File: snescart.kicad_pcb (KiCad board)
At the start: 2 copper layers, 101.6 x 37.3 mm, 7 parts, among them P1 CASSETTE, U1 27C080

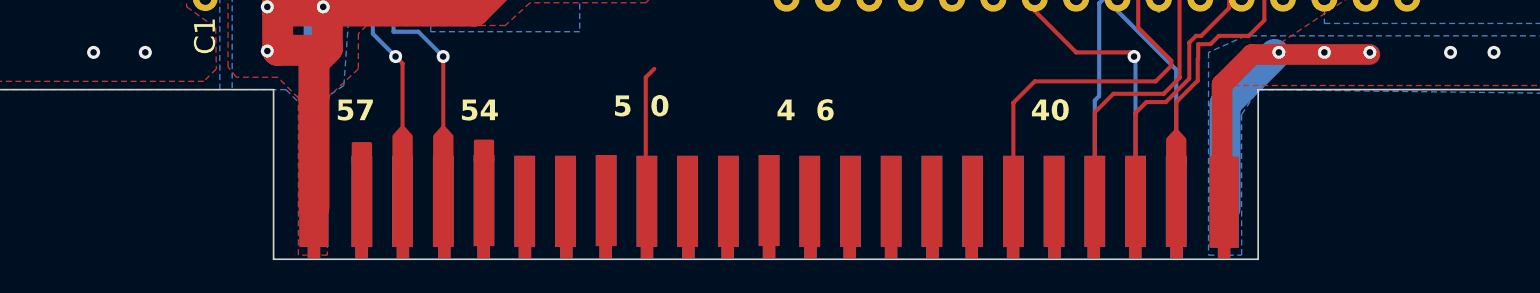
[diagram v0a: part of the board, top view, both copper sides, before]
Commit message: imperial mil cart edge
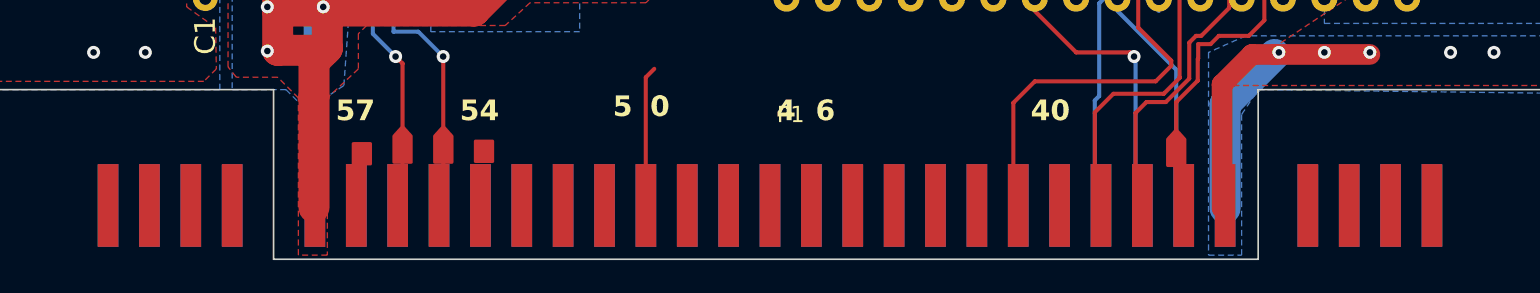
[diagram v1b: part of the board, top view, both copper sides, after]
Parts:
- P1: footprint Library:CartEdge -> Library:ImperialCart
- moved P1 1.51 mm to (146.3, 144.0)
